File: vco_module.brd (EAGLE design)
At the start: 14.3 x 26.3 mm, 11 parts, among them U1 MAX2606

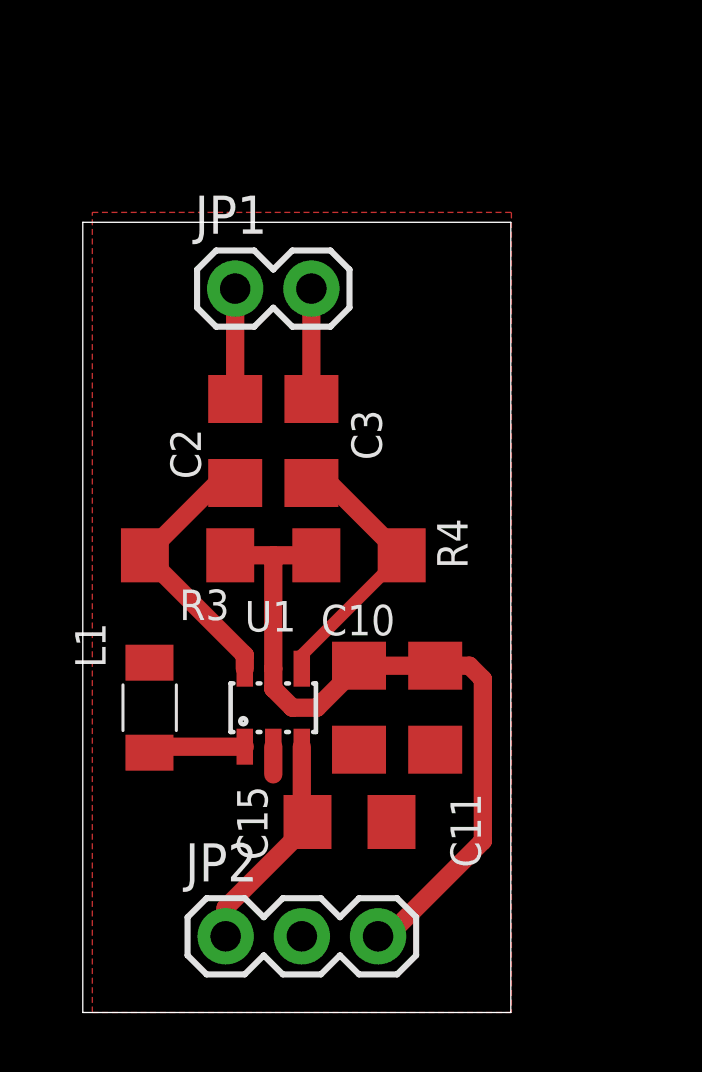
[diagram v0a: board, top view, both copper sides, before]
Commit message: final changes to unused external boards
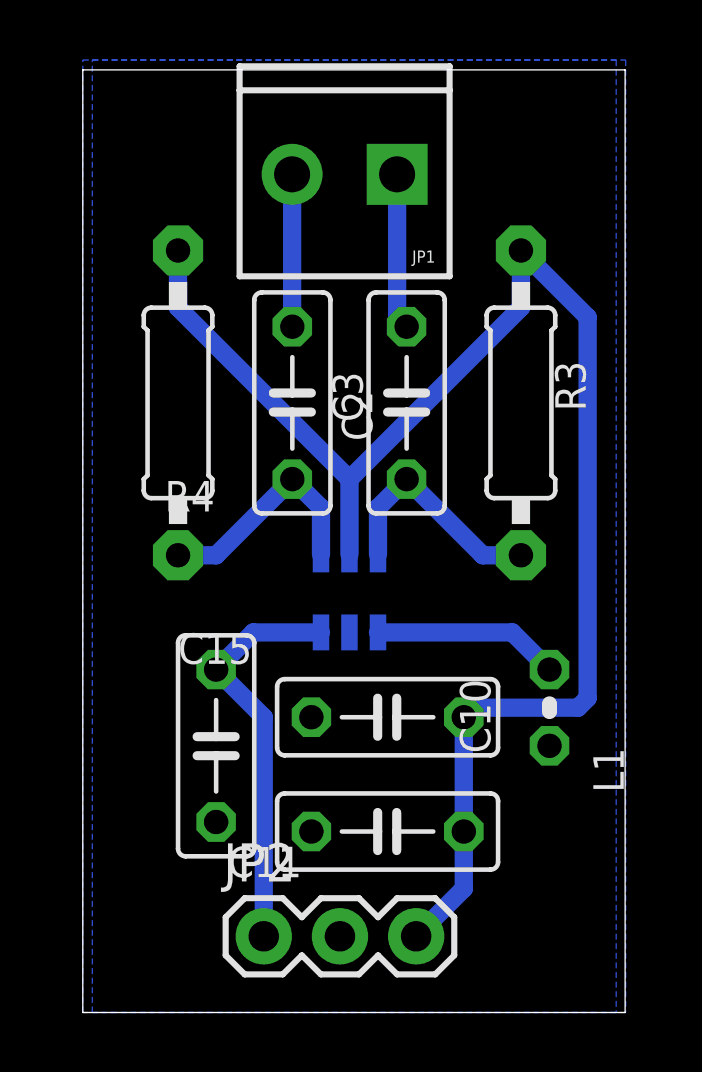
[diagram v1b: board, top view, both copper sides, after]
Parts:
- C10, C11, C15, C2, C3: device adafruit:C1206 -> adafruit:C050-025X075
- JP1: device sparkfun:1X02 -> sparkfun:SCREWTERMINAL-3.5MM-2
- L1: device resistor:L3216C -> resistor:0204V
- R3, R4: device adafruit:R1206 -> adafruit:0207/10
- moved L1 13.3 mm to (15.6, 10.2), turned to 90 degrees
- moved R3 12.2 mm to (14.6, 20.3), turned to 270 degrees
- moved R4 7.89 mm to (3.17, 20.3), turned to 270 degrees
- moved JP1 6.61 mm to (10.5, 27.9), turned to 180 degrees
- moved C2 5.85 mm to (10.8, 20.3)
- moved C15 5.12 mm to (4.45, 8.89), turned to 270 degrees
- moved U1 4.58 mm to (8.89, 14.0), flipped to the bottom
- moved C11 4.42 mm to (10.2, 6.03), turned to 180 degrees
- moved C3 1.42 mm to (6.99, 20.3)
- moved JP2 1.27 mm to (6.03, 2.54)
- moved C10 1.00 mm to (10.2, 9.84), turned to 180 degrees
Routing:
- net VCC: track 25.7 -> 50.7 mm
- net SIGNAL: track 10.5 -> 13.6 mm
- net N$24: track 3.26 -> 6.23 mm
- net N$39: track 3.68 -> 5.21 mm
- net N$52: track 3.68 -> 5.08 mm
- net N$35: track 9.17 -> 7.77 mm
- net N$33: track 9.17 -> 7.77 mm
- net GND: track 0.92 -> 0.00 mm
- added copper zone on layer 16, net GND
- added copper zone on layer 16, net N$1
- removed copper zone on layer 1, net GND
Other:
- board size 14.3 x 26.3 mm -> 18.1 x 31.4 mm
